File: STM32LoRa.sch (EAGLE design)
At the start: 40 parts, among them IC1 CMWX1ZZABZ-078, J3 USB_MINI-B_SMT, J4 Qwiic Right Angle, J7 U.FL, Q1 2.5A/30V/105mΩ, U1 TS3A4751PWR, U2 LTC3106EFE#PBF

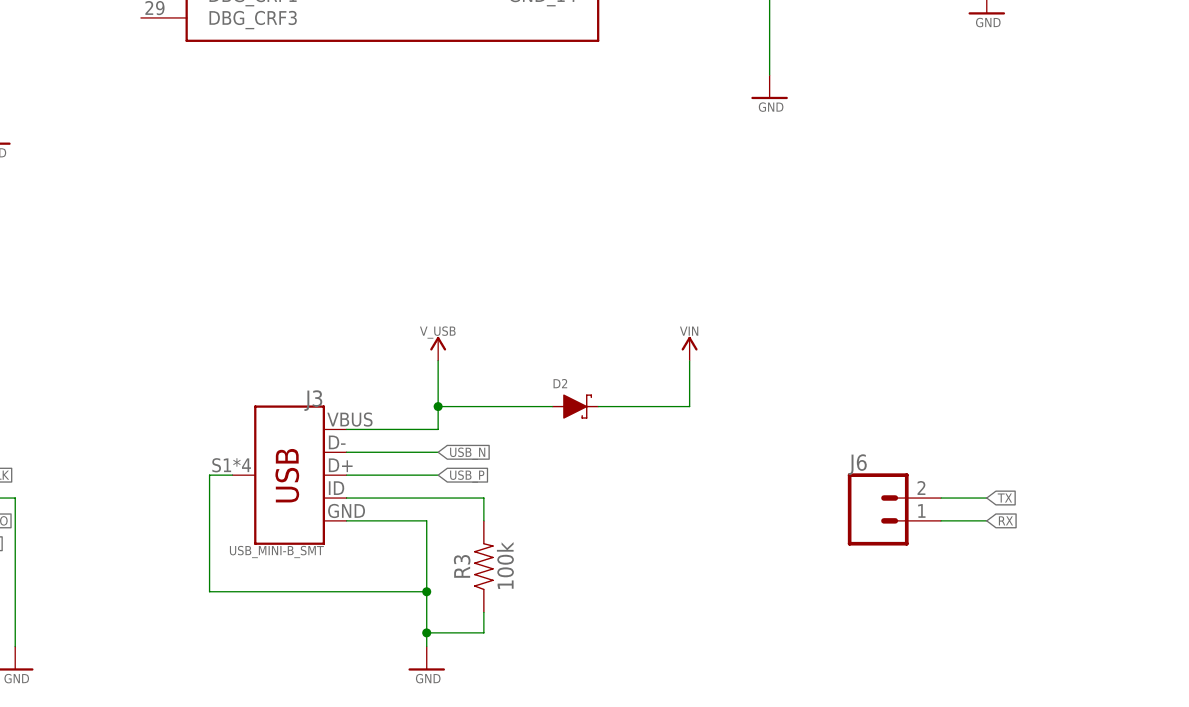
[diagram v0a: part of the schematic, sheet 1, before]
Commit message: File check in
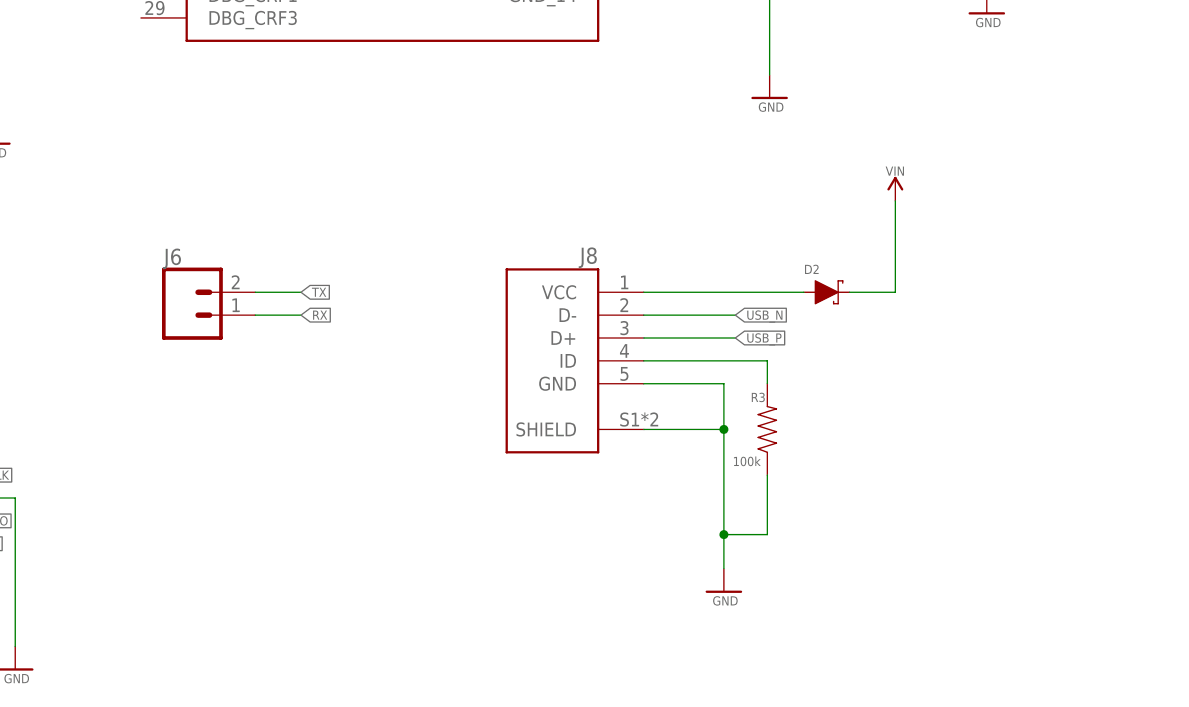
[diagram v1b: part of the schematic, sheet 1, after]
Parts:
- removed J3: USB_MINI-B_SMT, SparkFun-Connectors:USB_MINI-B_SMT
- added C16, C17: 0.1uF, SparkFun-Capacitors:0.1UF-0603-25V-(+80/-20%)
- added J8: USB3131-30-0230-A_REVB, USB3131-30-0230-A_REVB:USB3131-30-0230-A_REVB
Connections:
- removed net N$7: J3.ID, R3.2
- removed net V_USB: D2.A, J3.VBUS
- new net N$12: J8.ID, R3.2
- new net N$13: D2.A, J8.VCC
- net GND: now also C16.1, C17.1, J8.GND, J8.SHIELD; no longer J3.GND, J3.SHIELD
- net USB_N: now also J8.D-; no longer J3.D-
- net USB_P: now also J8.D+; no longer J3.D+
- net VCC_1: now also C16.2, C17.2
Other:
- moved on the sheet: D2, J5, J6, R3
